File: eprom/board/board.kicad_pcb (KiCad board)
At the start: 2 copper layers, 66.4 x 62.7 mm, 21 parts, among them J1 GPIO, J2 PWR, Q1 2N3904, Q2 BS250, U1 8755A, U2 MC33063AP

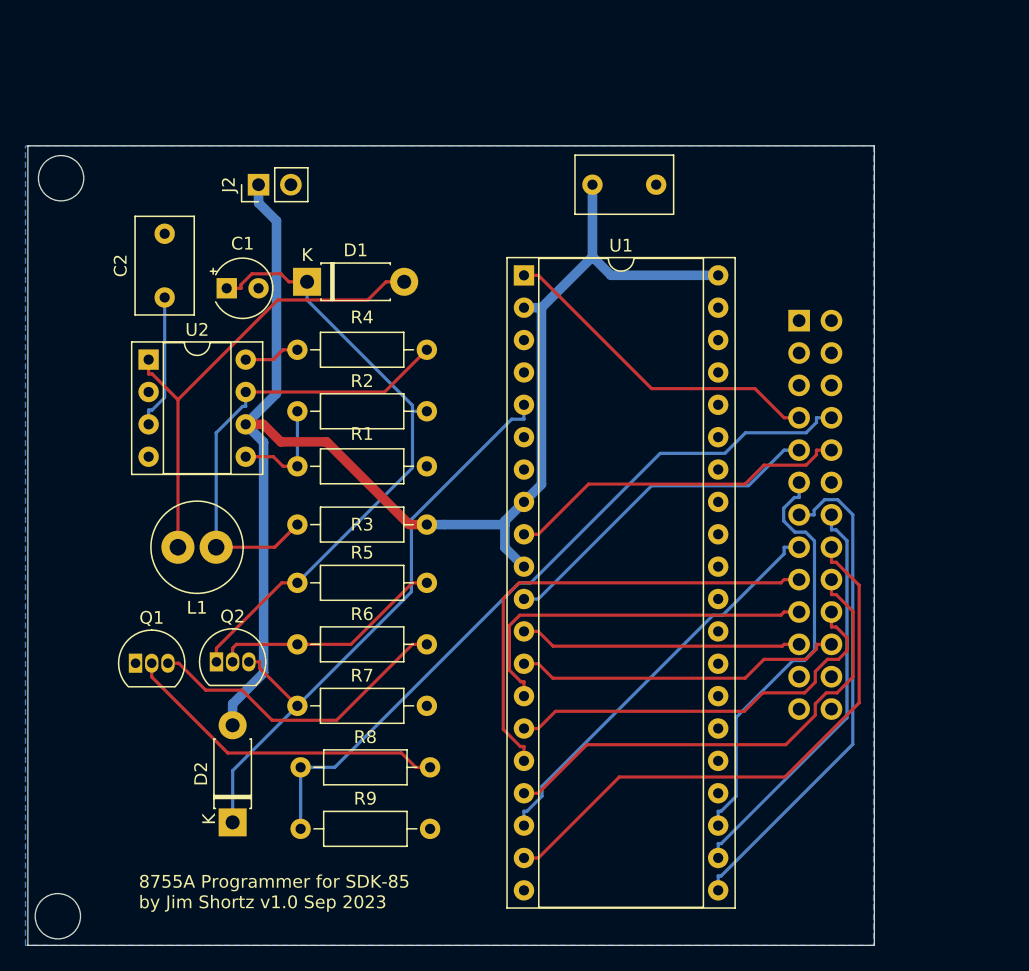
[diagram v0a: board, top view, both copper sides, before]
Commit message: Production version
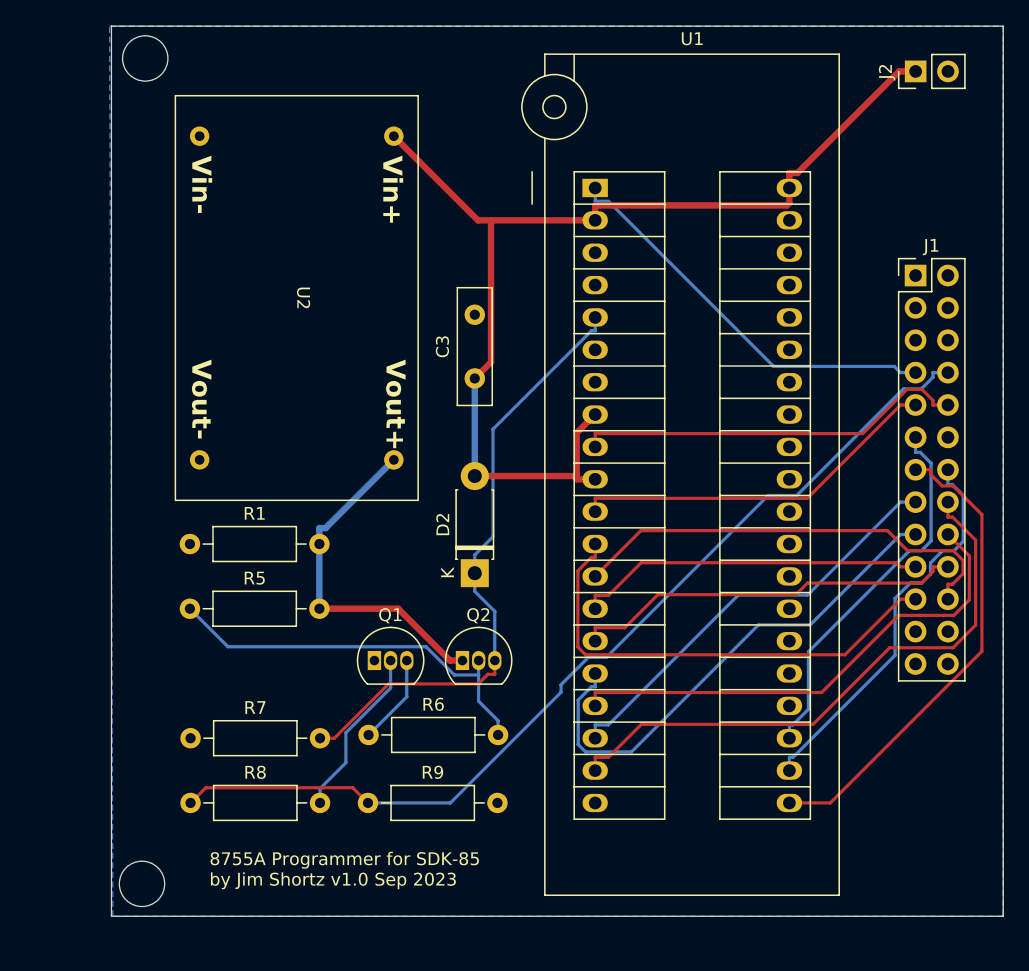
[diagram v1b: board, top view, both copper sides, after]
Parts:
- removed C1: 47uF, Capacitor_THT:CP_Radial_Tantal_D4.5mm_P2.50mm
- removed C2: 330pF, Capacitor_THT:C_Disc_D7.5mm_W4.4mm_P5.00mm
- removed D1: 1N5819, Diode_THT:D_DO-41_SOD81_P7.62mm_Horizontal
- removed L1: 100uH, Inductor_THT:L_Radial_D7.0mm_P3.00mm
- removed R2: 82K, Resistor_THT:R_Axial_DIN0207_L6.3mm_D2.5mm_P10.16mm_Horizontal
- removed R3: 0.68, Resistor_THT:R_Axial_DIN0207_L6.3mm_D2.5mm_P10.16mm_Horizontal
- removed R4: 180, Resistor_THT:R_Axial_DIN0207_L6.3mm_D2.5mm_P10.16mm_Horizontal
- C3: footprint Capacitor_THT:C_Disc_D7.5mm_W4.4mm_P5.00mm -> Capacitor_THT:C_Disc_D9.0mm_W2.5mm_P5.00mm
- J1: footprint Connector_PinSocket_2.54mm:PinSocket_2x13_P2.54mm_Vertical -> Connector_PinHeader_2.54mm:PinHeader_2x13_P2.54mm_Vertical; moved to F.Cu
- R1: value 4.3K -> 1500
- U1: footprint Package_DIP:DIP-40_W15.24mm_Socket -> Socket:3M_Textool_240-1288-00-0602J_2x20_P2.54mm
- U2: value MC33063AP -> ~; footprint Package_DIP:DIP-8_W7.62mm_Socket -> parts:MT3608_Module
- moved J2 52.3 mm to (198.1, 35.1)
- moved D2 27.3 mm to (163.5, 74.4)
- moved R1 19.6 mm to (141.2, 72.1), turned to 0 degrees
- moved Q2 19.3 mm to (162.6, 81.3)
- moved Q1 18.7 mm to (155.7, 81.3)
- moved C3 17.8 mm to (163.5, 59.1), turned to 90 degrees
- moved U2 12.6 mm to (149.6, 52.8), turned to -90 degrees
- moved J1 9.80 mm to (198.1, 51.1), turned to 0 degrees
- moved R8 9.08 mm to (141.2, 92.5)
- moved R6 9.04 mm to (155.2, 87.1)
- moved U1 8.84 mm to (173.0, 44.2)
- moved R7 8.76 mm to (141.2, 87.4)
- moved R5 8.67 mm to (141.2, 77.2)
- moved R9 5.66 mm to (155.1, 92.5)
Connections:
- net VDD_EN renamed /VDD_EN
- net ~{RD} renamed /~{RD}
- D2 pad 1: VDD -> Net-(D2-K)
- Q2 pad 3: VDD -> Net-(D2-K)
- R1 pad 2: Net-(U2-Vfb) -> /+25V
- R5 pad 1: /+25V -> Net-(Q2-G)
- R5 pad 2: Net-(Q2-G) -> /+25V
- R6 pad 1: Net-(Q2-G) -> Net-(Q1-C)
- R6 pad 2: Net-(Q1-C) -> Net-(Q2-G)
- R7 pad 1: VDD -> GND
- R7 pad 2: GND -> Net-(D2-K)
- U1 pad 5: VDD -> Net-(D2-K)
- U2 pad 1: Net-(D1-A) -> GND
- U2 pad 3: Net-(U2-TC) -> /+25V
- U2 pad 4: GND -> VCC
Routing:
- net Net-(D2-K): track 0.00 -> 48.5 mm
- net VDD: track 48.3 -> 0.00 mm
- net Net-(D1-A): track 37.4 -> 0.00 mm
- net Net-(U2-Ipk): track 36.0 -> 0.00 mm
- net VCC: track 114.5 -> 86.3 mm
- net /+25V: track 48.7 -> 27.3 mm
- net Net-(Q1-C): track 24.6 -> 7.08 mm
- net /VDD_EN: track 58.1 -> 75.0 mm
- net /AD0: track 22.1 -> 37.4 mm
- net Net-(Q2-G): track 18.4 -> 31.3 mm
- net Net-(Q1-B): track 25.9 -> 13.5 mm
- net Net-(U2-TC): track 10.6 -> 0.00 mm
- net /AD1: track 25.9 -> 35.1 mm
- net Net-(U2-Vfb): track 8.68 -> 0.00 mm
- net PROG: track 26.2 -> 31.8 mm
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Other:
- board size 66.4 x 62.7 mm -> 70 x 69.8 mm
